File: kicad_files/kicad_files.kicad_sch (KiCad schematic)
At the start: 13 parts, among them J1 Battery Connection, J2 Servo Connection, J3 DC Motor Connection, J4 Washout Ultrasonic Sensor Con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, J5 Water Sensor Connection, J6 DC Motor Connection, J7 Larvicide Level Ultrasonic Se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

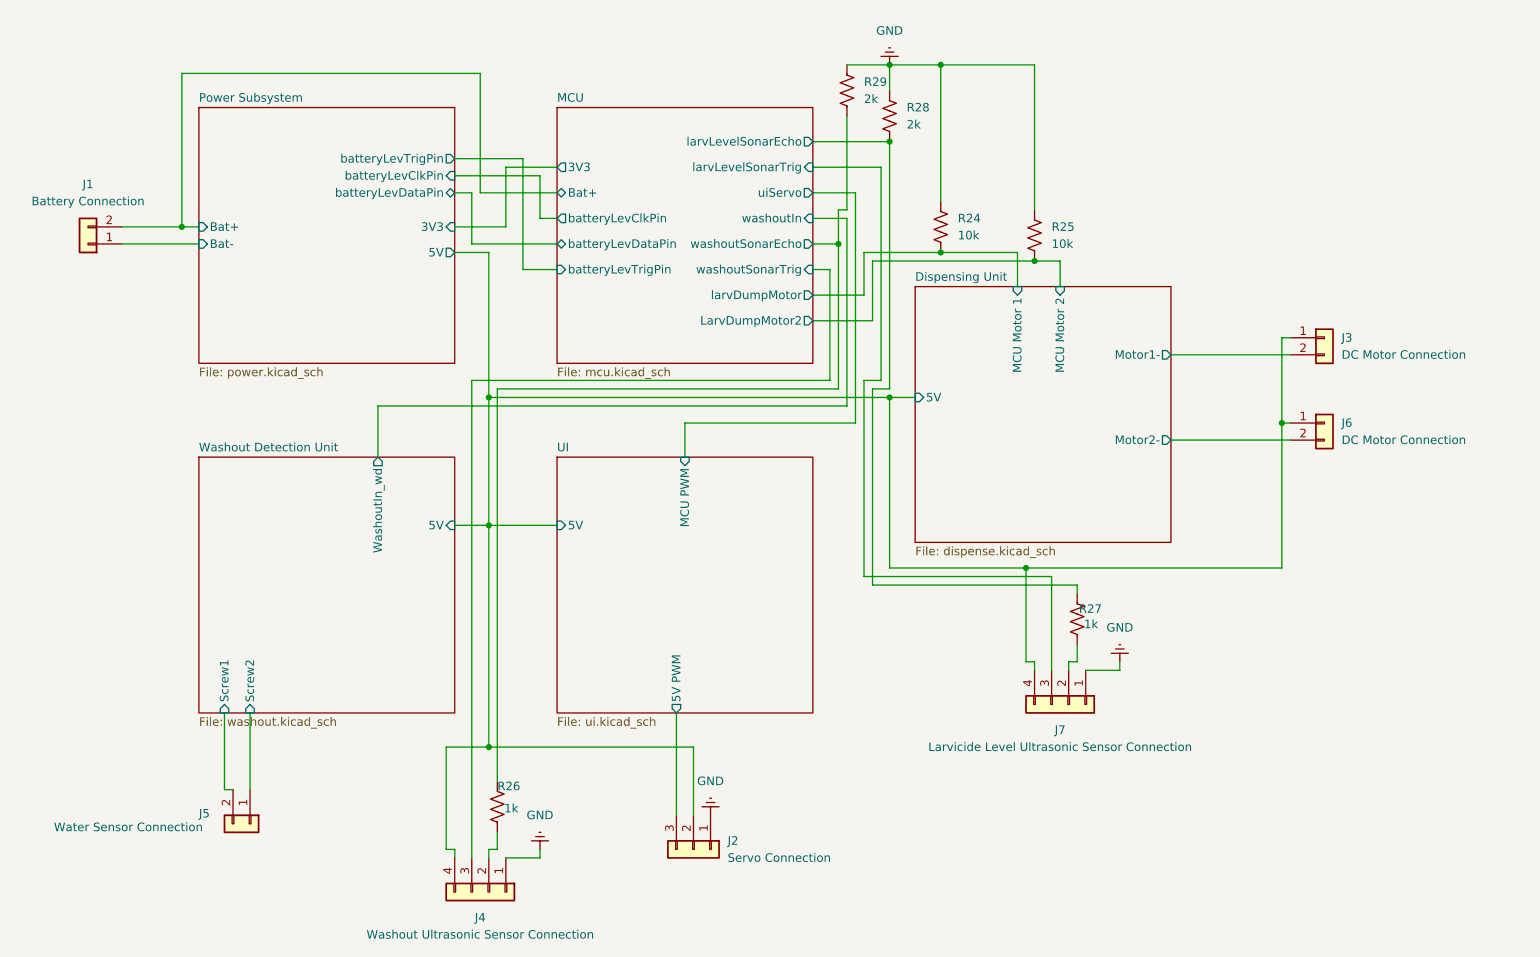
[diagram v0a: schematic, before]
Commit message: minor changes
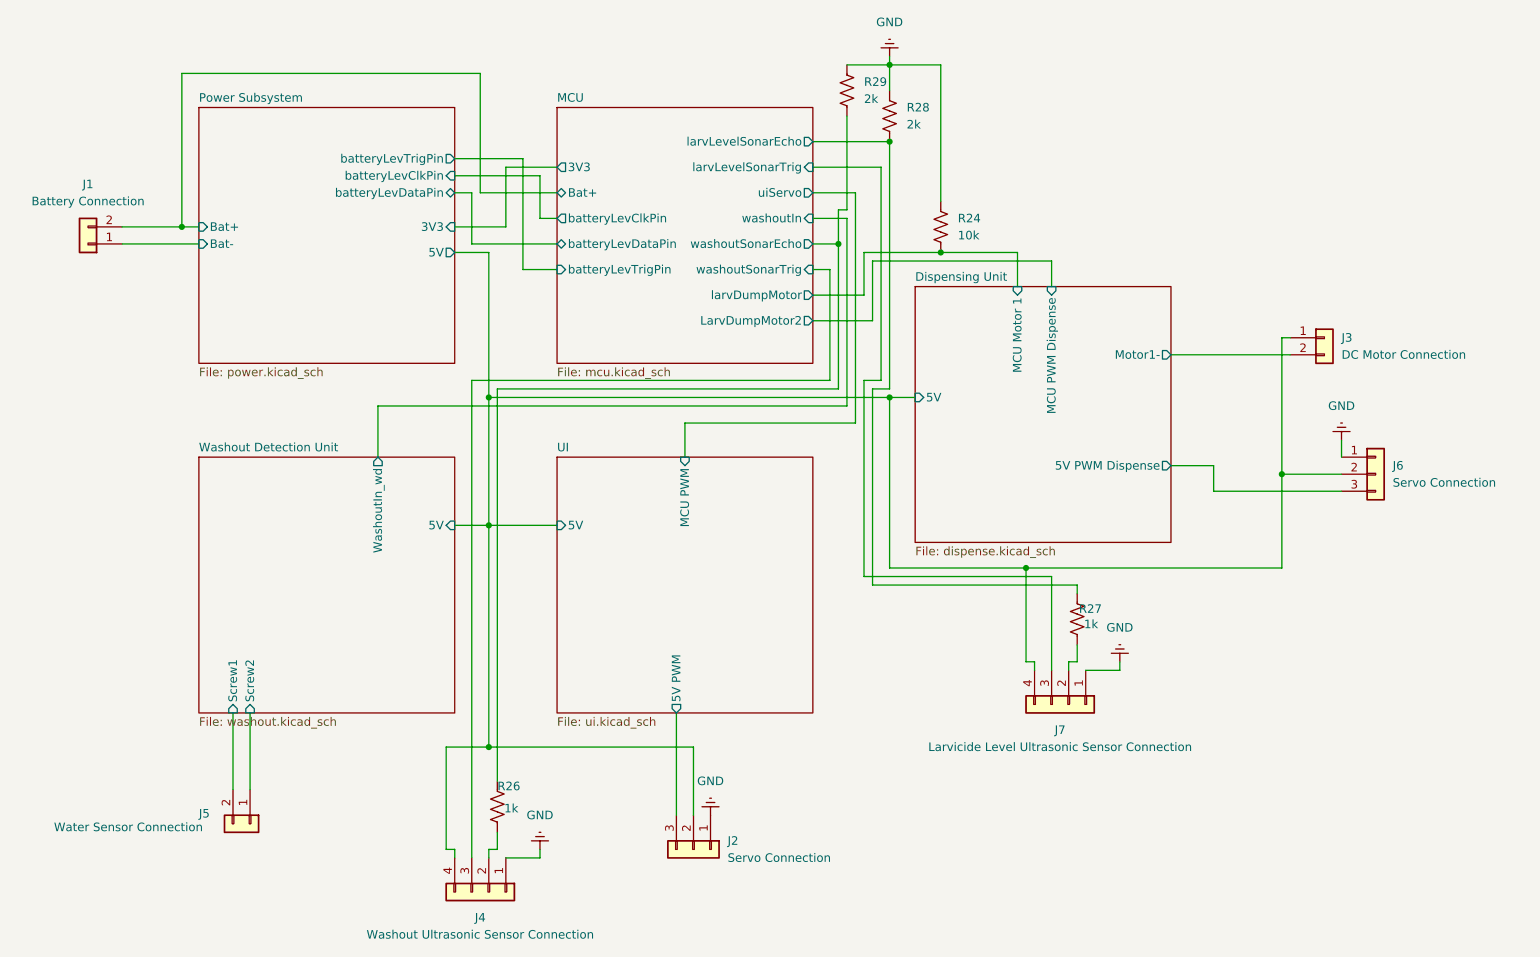
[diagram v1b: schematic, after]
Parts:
- removed J6: DC Motor Connection, symbol Connector_Generic:Conn_01x02
- removed R25: 10k, symbol Device:R_US
- added J6: Servo Connection, symbol Connector_Generic:Conn_01x03
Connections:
- net Dispensing Unit/5V: now also J6.2 (Pin_2)
- net GND: now also J6.1 (Pin_1)
- new net Dispensing Unit/5V PWM Dispense: J6.3 (Pin_3)
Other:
- sheet Dispensing Unit ports: added 5V PWM Dispense, MCU PWM Dispense; removed MCU Motor 2, Motor2-
